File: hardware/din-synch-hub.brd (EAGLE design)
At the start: 140.7 x 20.2 mm, 47 parts, among them IC1 6N138, IC2 PIC12F1822SO08, IC3 4050D, IC4 REG1117, IC6 4050D, X1 DIN5PIN, X2 DIN5PIN, X3 DIN5PIN, X4 DIN5PIN, X5 DIN5PIN, X6 DIN5PIN

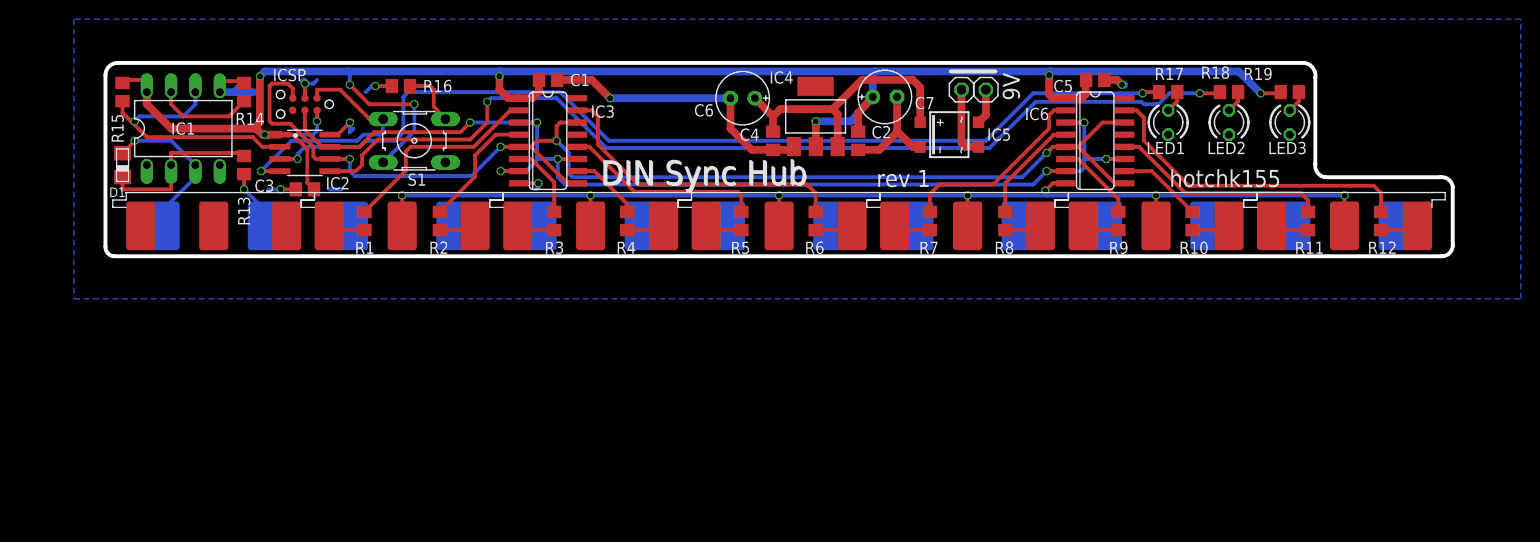
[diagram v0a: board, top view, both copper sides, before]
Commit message: updates
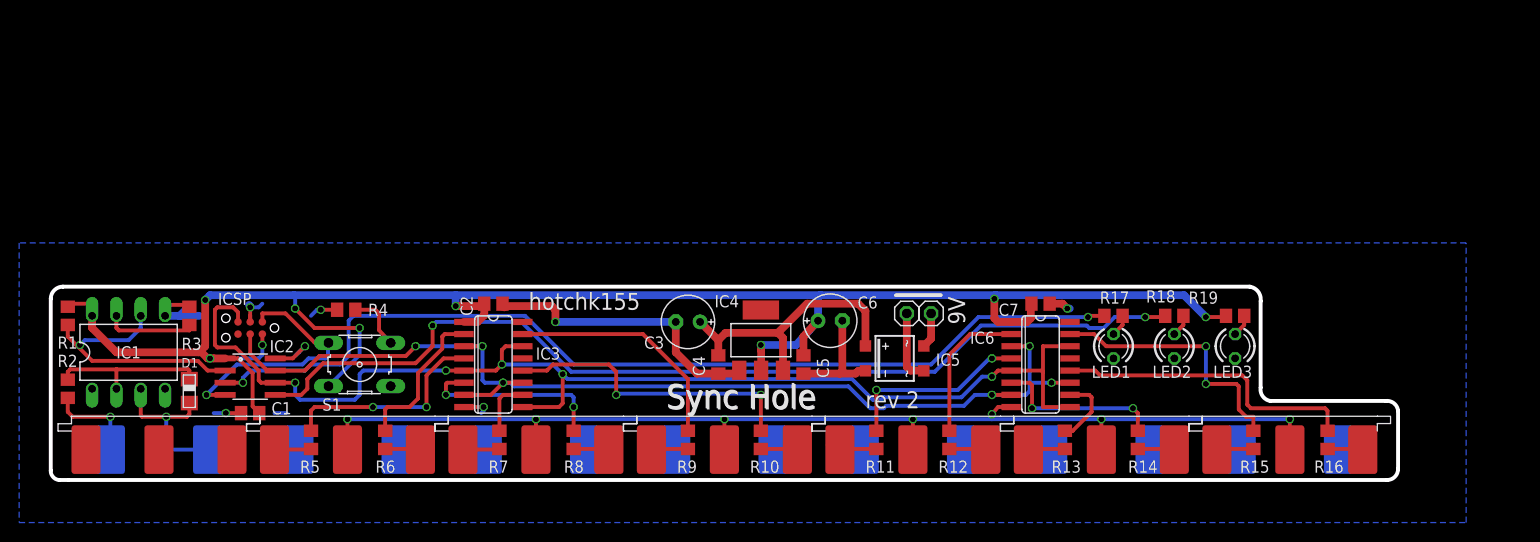
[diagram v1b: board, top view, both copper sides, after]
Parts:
- C3: device rcl:C0805 -> rcl:E2,5-6E
- C7: device rcl:E2,5-6E -> rcl:C0805
- moved R15 123.6 mm to (125.7, 4.32), turned to 270 degrees
- moved R16 103.6 mm to (133.5, 4.32), turned to 270 degrees
- moved R14 100.2 mm to (113.7, 4.32), turned to 270 degrees
- moved R13 90.4 mm to (106.0, 4.32), turned to 270 degrees
- moved R10 50.5 mm to (74.3, 4.32)
- moved R11 50.5 mm to (86.4, 4.32)
- moved R12 50.5 mm to (94.0, 4.32)
- moved R8 50.5 mm to (54.7, 4.32)
- moved R5 50.4 mm to (27.3, 4.32)
- moved R6 50.4 mm to (35.1, 4.32)
- moved R9 50.4 mm to (66.7, 4.32)
- moved R7 50.4 mm to (47.0, 4.32)
- moved C1 46.7 mm to (21.0, 7.11), turned to 180 degrees
- moved R2 42.6 mm to (1.91, 9.65), turned to 90 degrees
- moved C5 42.6 mm to (78.7, 12.2), turned to 270 degrees
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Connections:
- net GND: now also C3.-, C5.2, C7.1, R3.2, R4.1; no longer C3.2, C5.1, C7.-, R14.2, R16.1
- net IN: now also R1.1; no longer R15.1
- net N$1: now also R6.1; no longer R1.1
- net N$10: now also R10.2; no longer R5.2
- net N$11: now also R9.2; no longer R6.2
- net N$12: now also R9.1; no longer R6.1
- net N$13: now also R12.1; no longer R7.1
- net N$14: now also R12.2; no longer R7.2
- net N$15: now also R11.1; no longer R8.1
- net N$16: now also R11.2; no longer R8.2
- net N$17: now also R14.1; no longer R9.1
- net N$18: now also R14.2; no longer R9.2
- net N$19: now also R13.1; no longer R10.1
- net N$2: now also R6.2; no longer R1.2
- net N$20: now also R13.2; no longer R10.2
- net N$21: now also R16.1; no longer R11.1
- net N$22: now also R16.2; no longer R11.2
- net N$23: now also R15.2; no longer R12.2
- net N$24: now also R15.1; no longer R12.1
- net N$26: now also R2.1; no longer R13.1
- net N$27: now also R2.2; no longer R13.2
- net N$29: now also R3.1; no longer R14.1
- net N$3: now also R5.1; no longer R2.1
- net N$30: now also R4.2; no longer R16.2
- net N$32: now also C3.+; no longer C6.+
- net N$4: now also R5.2; no longer R2.2
- net N$5: now also R8.1; no longer R3.1
- net N$6: now also R8.2; no longer R3.2
- net N$7: now also R7.1; no longer R4.1
- net N$8: now also R7.2; no longer R4.2
- net N$9: now also R10.1; no longer R5.1
- net VCC: now also C5.1, C6.+, C7.2, R1.2; no longer C3.1, C5.2, C7.+, R15.2
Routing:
- net N$5: track 7.82 -> 20.0 mm, vias 0 -> 2
- net N$9: track 20.9 -> 31.9 mm, vias 0 -> 2
- net N$21: track 22.7 -> 32.2 mm
- net N$3: track 12.9 -> 22.3 mm, vias 0 -> 2
- net N$17: track 8.56 -> 17.8 mm, vias 0 -> 2
- net N$15: track 11.4 -> 19.7 mm, vias 0 -> 2
- net N$12: track 32.1 -> 24.6 mm
- net N$24: track 33.7 -> 27.9 mm, vias 0 -> 2
- net N$13: track 20.5 -> 15.3 mm
- net N$1: track 21.7 -> 16.9 mm
- net N$26: track 6.19 -> 9.55 mm
- net CLK: track 115.1 -> 112.2 mm, vias 7 -> 6
- net N$16: track 3.87 -> 6.74 mm
- net GND: track 191.3 -> 194.0 mm
- net RUN: track 123.9 -> 126.5 mm, vias 4 -> 5
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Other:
- board text added: "Sync Hole"
- board text added: "rev 2"
- board text removed: "DIN Sync Hub"
- board text removed: "rev 1"
